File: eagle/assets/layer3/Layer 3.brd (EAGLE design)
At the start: 90 x 90 mm, 82 parts, among them Q2 AO3402, X1 SM06B-SRSS-TB, Y1 8MHz

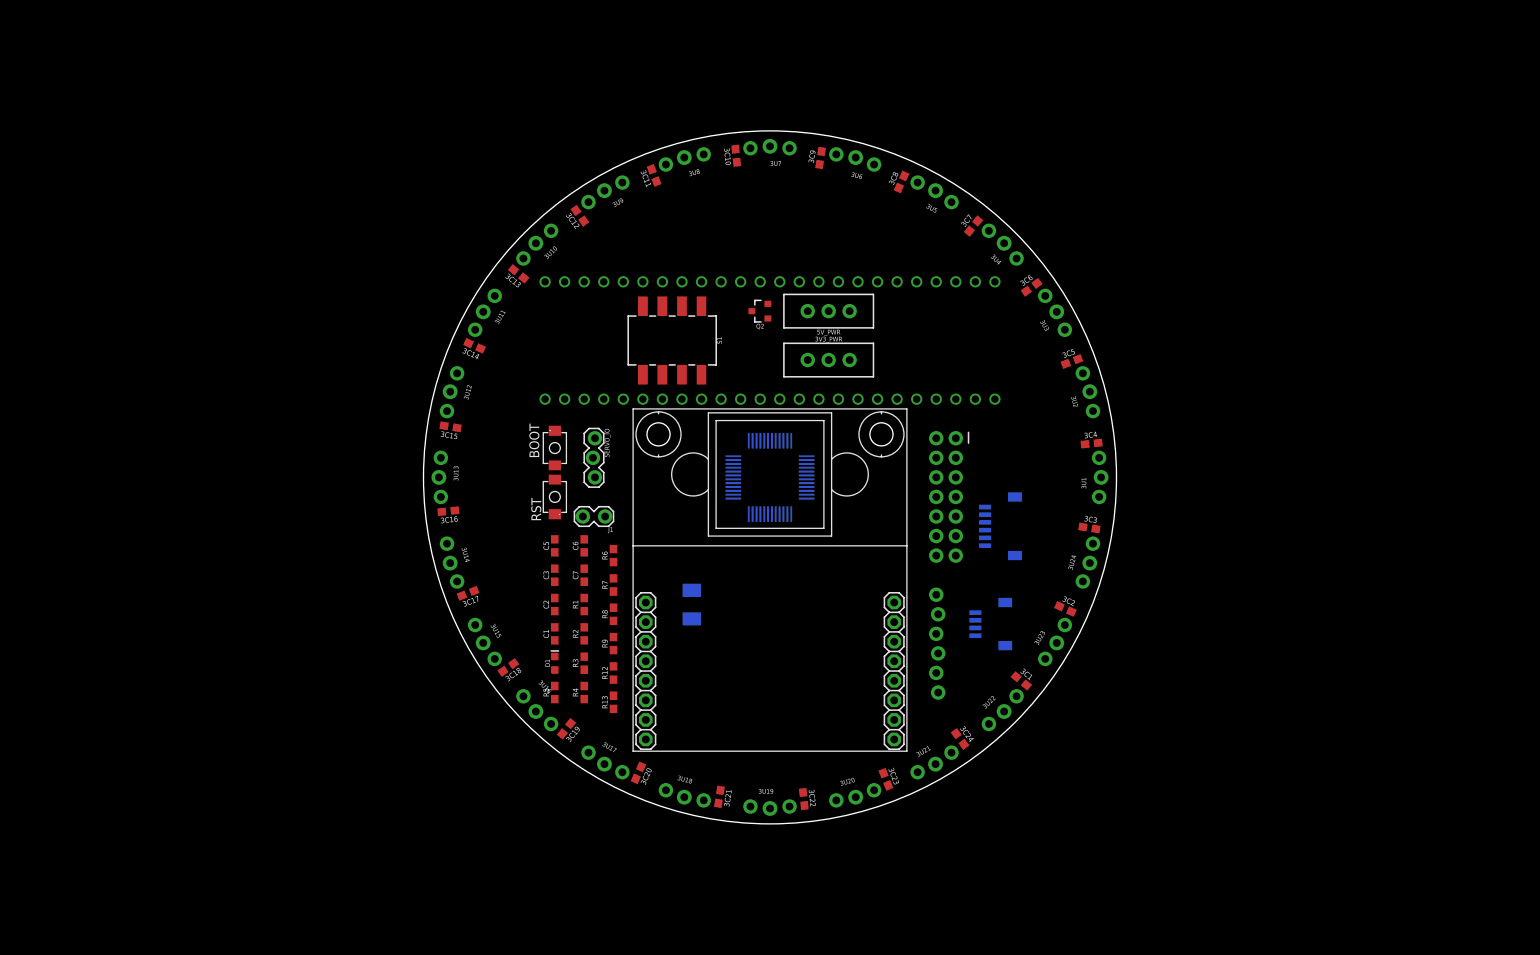
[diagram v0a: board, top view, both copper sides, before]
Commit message: eagle
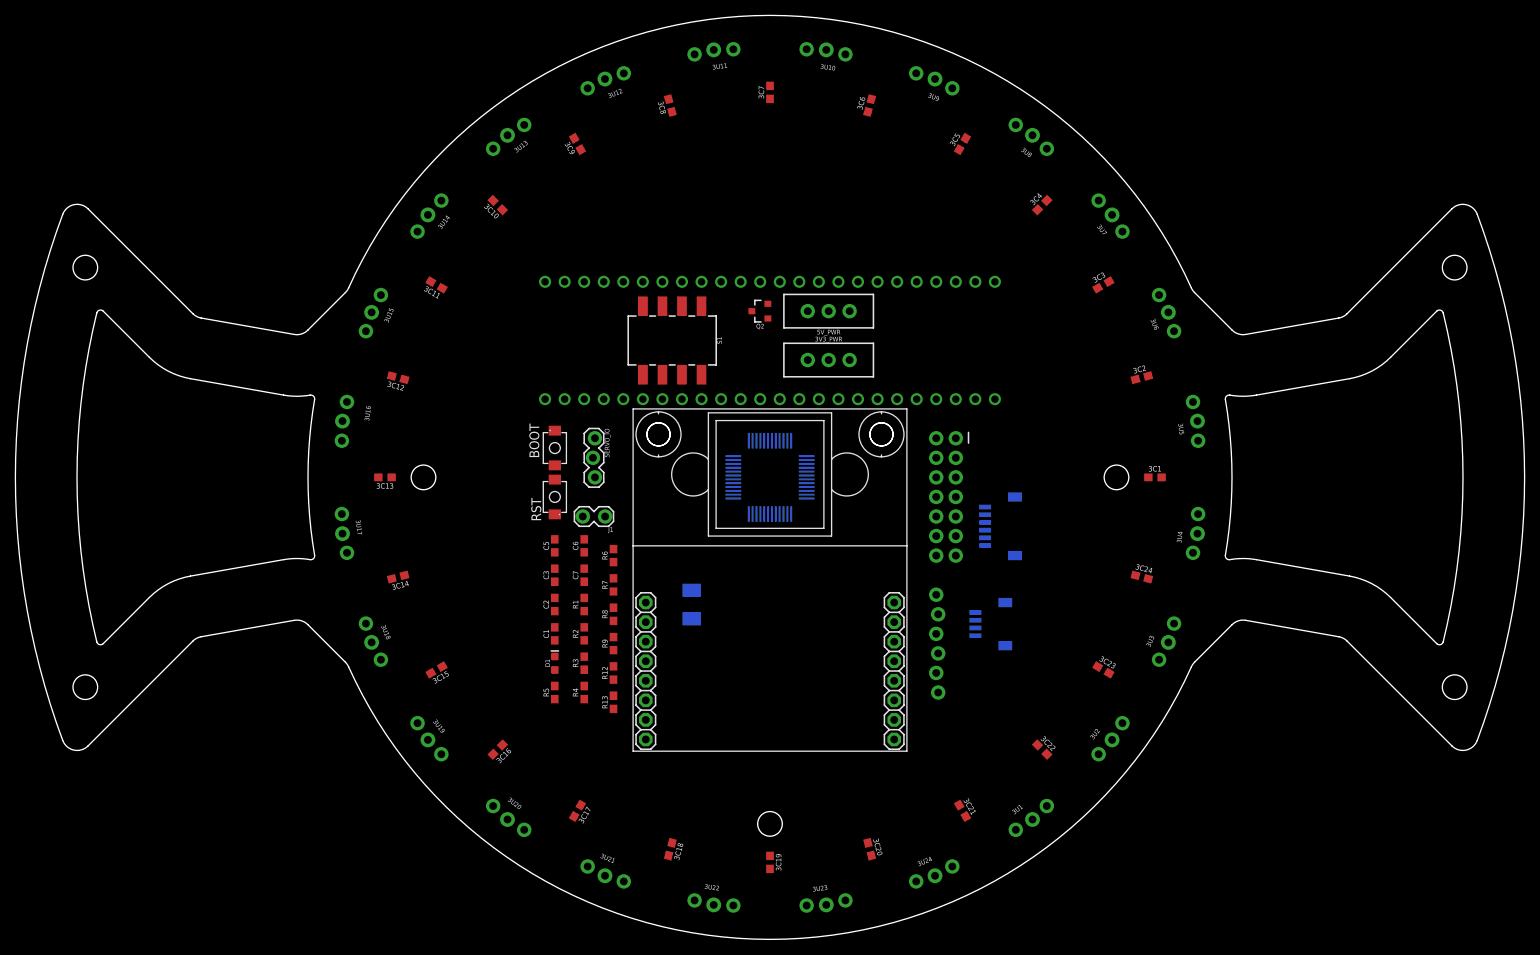
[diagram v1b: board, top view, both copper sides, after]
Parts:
- moved 3U11 45.3 mm to (-7.31, 55.5), turned to 97.5 degrees
- moved 3U17 45.3 mm to (-55.5, -7.31), turned to 187.5 degrees
- moved 3U23 45.3 mm to (7.31, -55.5), turned to 277.5 degrees
- moved 3U5 45.3 mm to (55.5, 7.31), turned to 7.5 degrees
- moved 3U14 45.3 mm to (-44.4, 34.1), turned to 142.5 degrees
- moved 3U2 45.3 mm to (44.4, -34.1), turned to 322.5 degrees
- moved 3U20 45.3 mm to (-34.1, -44.4), turned to 232.5 degrees
- moved 3U8 45.3 mm to (34.1, 44.4), turned to 52.5 degrees
- moved 3U1 45.3 mm to (34.1, -44.4), turned to 307.5 degrees
- moved 3U13 45.3 mm to (-34.1, 44.4), turned to 127.5 degrees
- moved 3U19 45.3 mm to (-44.4, -34.1), turned to 217.5 degrees
- moved 3U7 45.3 mm to (44.4, 34.1), turned to 37.5 degrees
- moved 3U12 45.3 mm to (-21.4, 51.7), turned to 112.5 degrees
- moved 3U18 45.3 mm to (-51.7, -21.4), turned to 202.5 degrees
- moved 3U24 45.3 mm to (21.4, -51.7), turned to 292.5 degrees
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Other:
- board size 90 x 90 mm -> 196 x 120 mm
